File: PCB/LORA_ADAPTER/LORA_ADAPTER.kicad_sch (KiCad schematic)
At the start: 39 parts, among them J1 Conn_02x06_Odd_Even, J2 Conn_02x06_Odd_Even, J3 BM06B-SRSS-TBT(LF)(SN), J4 BM06B-SRSS-TBT(LF)(SN), J5 BM06B-SRSS-TBT(LF)(SN), J6 BM06B-SRSS-TBT(LF)(SN), J7 BM06B-SRSS-TBT(LF)(SN), J8 BM06B-SRSS-TBT(LF)(SN), J9 Battery, U2 TCA9534, U3 AP2112K-3.3, U4 AP2112K-3.3, U4 MCP73831-2-OT, U5 AP2112K-3.3, U6 AP2112K-3.3, U7 AP2112K-3.3, U8 AP2112K-3.3, U9 AP2112K-3.3

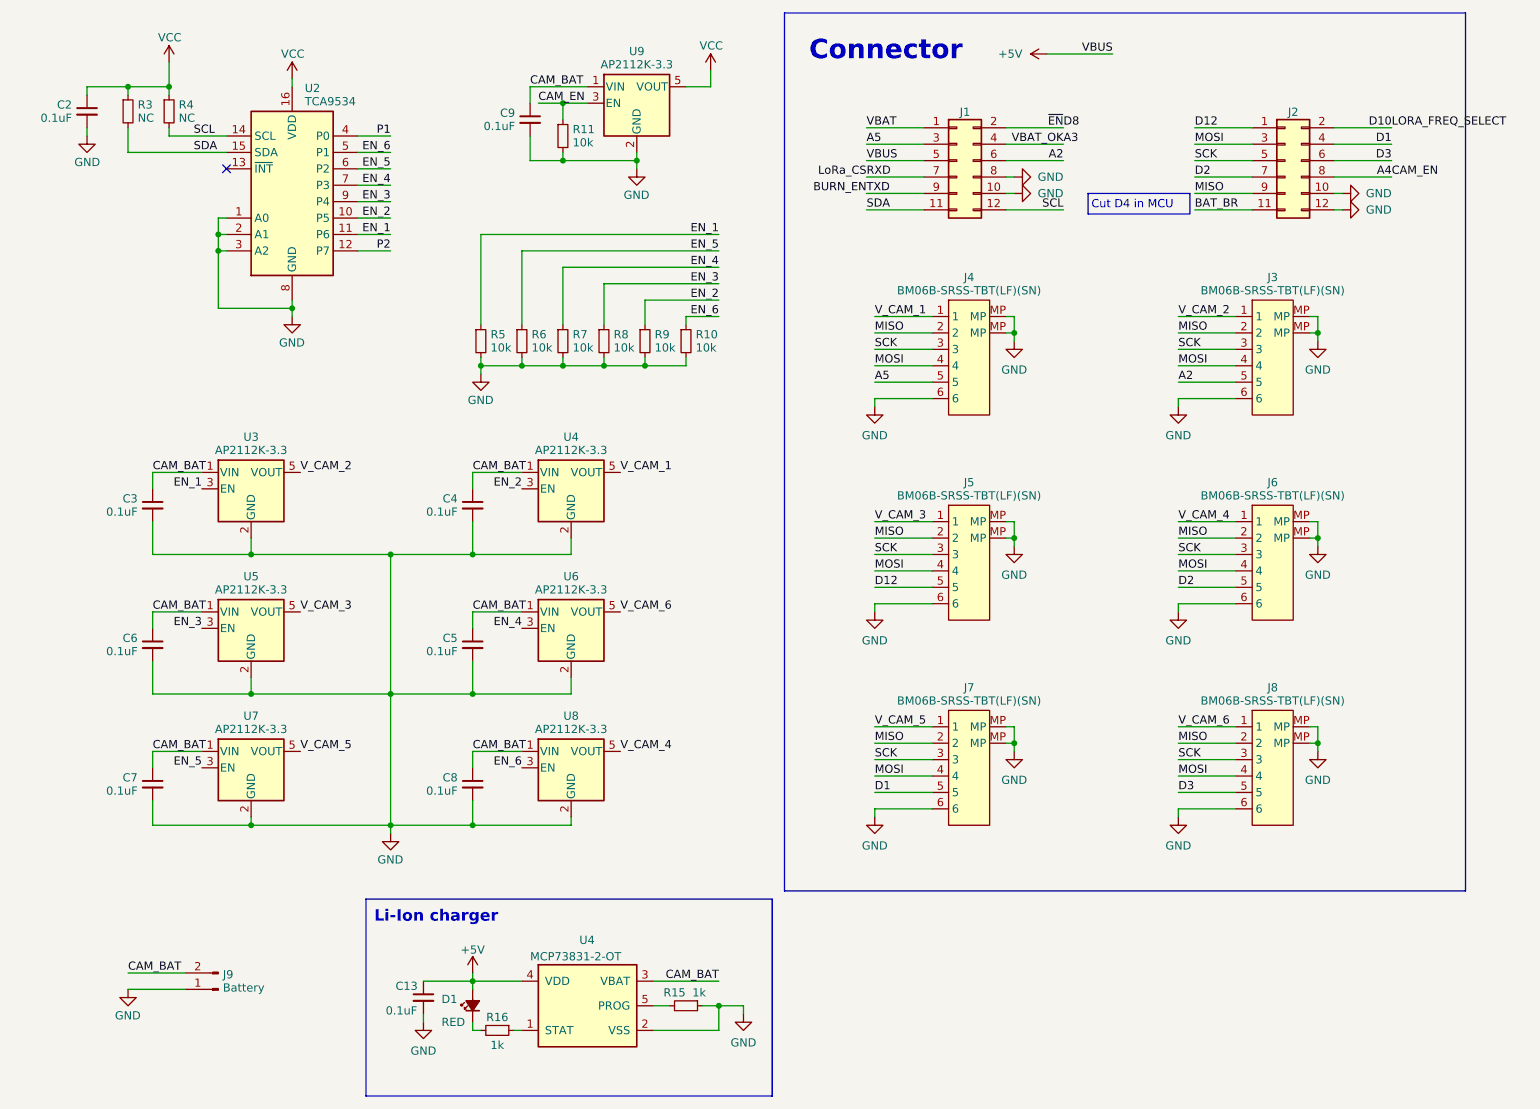
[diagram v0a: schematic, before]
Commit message: udated by FZ
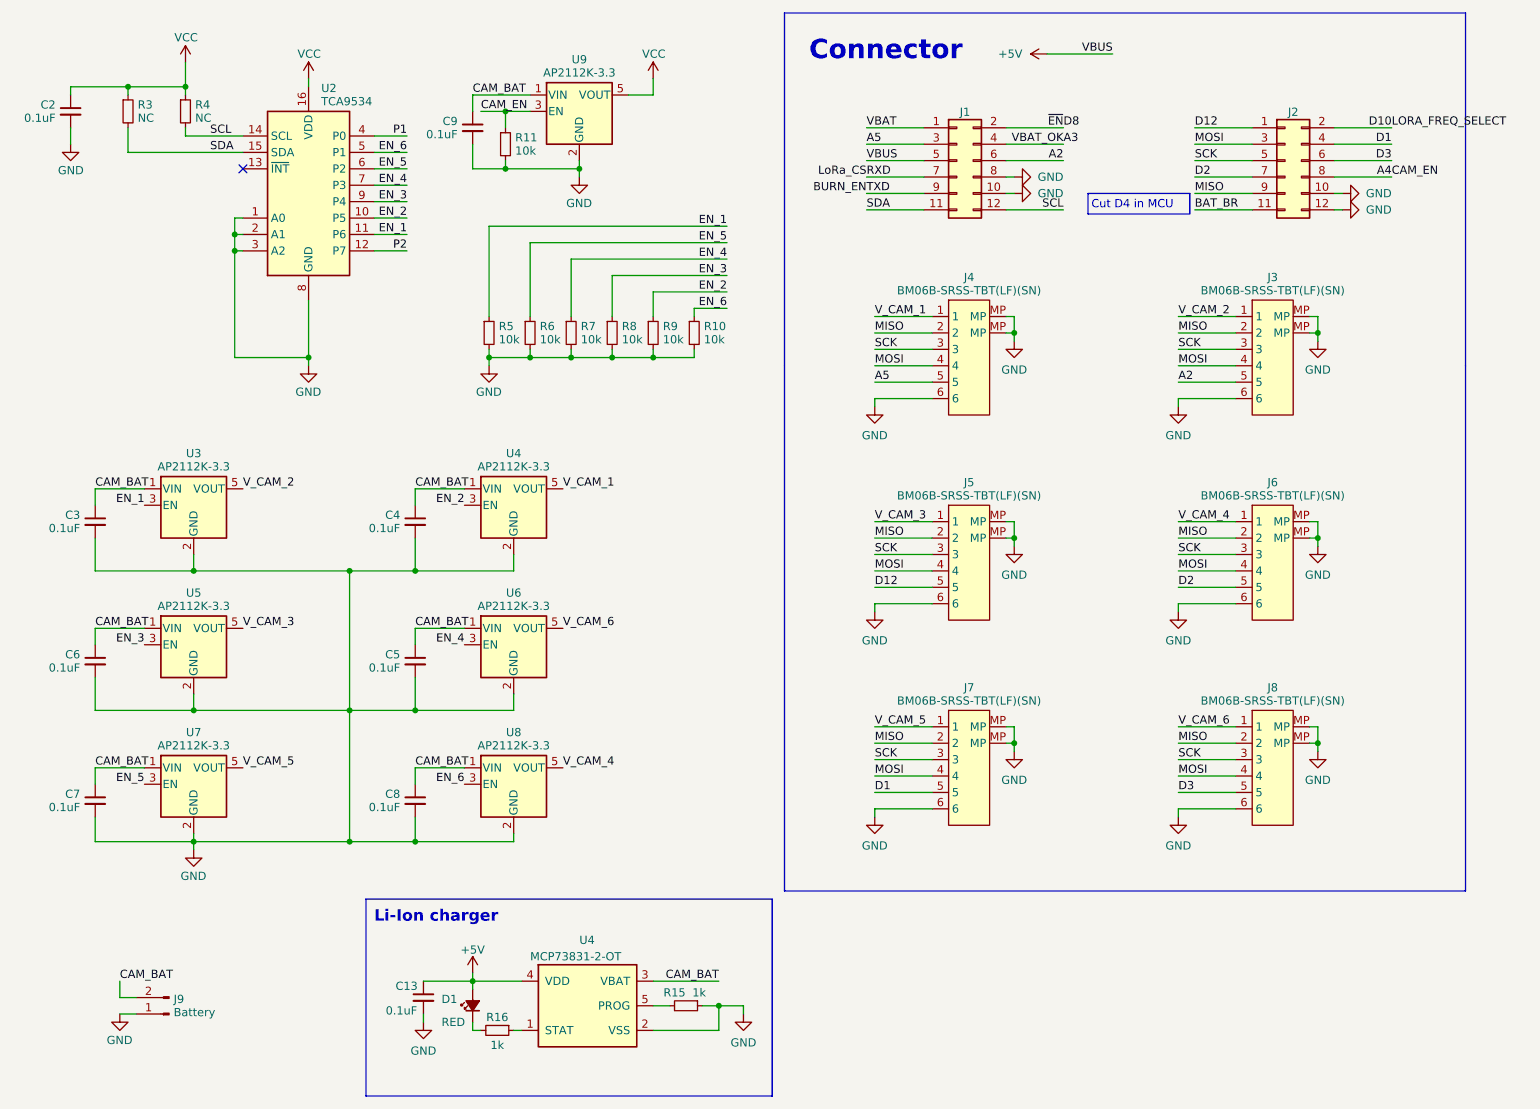
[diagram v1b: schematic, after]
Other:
- moved on the sheet: C2, C3, C4, C5, C6, C7, C8, C9, J9, R10, R11, R4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
